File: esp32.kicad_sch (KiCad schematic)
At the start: 52 parts, among them J2 Conn_01x05, SW1 Reset, SW2 BOOT, U15 MPR121QR2, U8 ESP32-S3R8, U9 W25Q128JVSIQ, Y1 40MHz

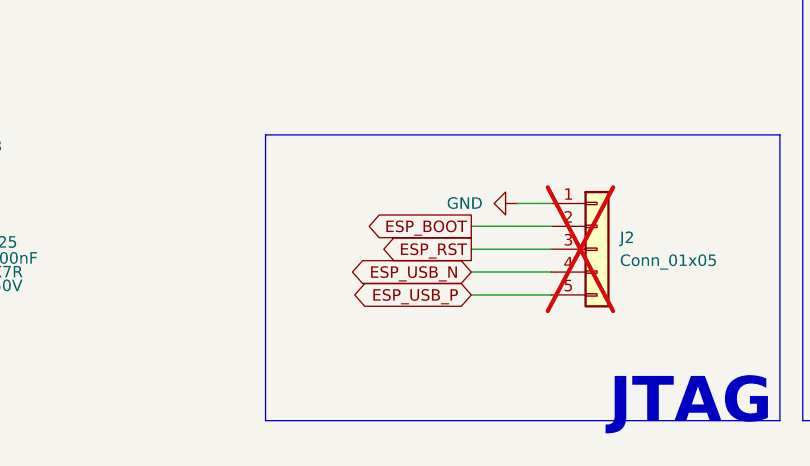
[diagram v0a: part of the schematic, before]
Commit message: WiP update
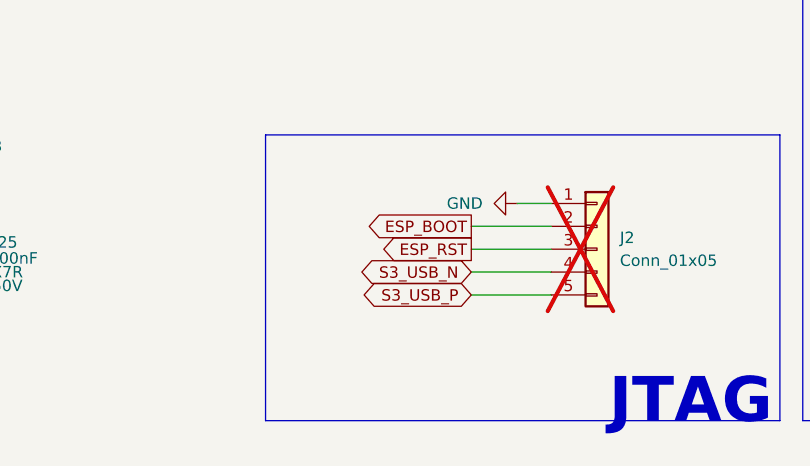
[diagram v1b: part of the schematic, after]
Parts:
- TP14, TP15, TP16: footprint TestPoint:TestPoint_Pad_2.5x2.5mm -> Onju:Touchpad
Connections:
- net ESP_USB_N is gone; now on net S3_USB_N: J2.4 (Pin_4)
- net ESP_USB_P is gone; now on net S3_USB_P: J2.5 (Pin_5)
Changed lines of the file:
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@@
 		)
 	)
-	(global_label "ESP_USB_N"
+	(global_label "S3_USB_N"
 		(shape bidirectional)
 		(at 106.68 264.16 180)
@@
 		)
 		(property "Intersheetrefs" "${INTERSHEET_REFS}"
-			(at 91.8793 264.16 0)
+			(at 93.0888 264.16 0)
 			(effects
 				(font
@@
 		)
 	)
-	(global_label "ESP_USB_P"
+	(global_label "S3_USB_P"
 		(shape bidirectional)
 		(at 106.68 266.7 180)
@@
 		)
 		(property "Intersheetrefs" "${INTERSHEET_REFS}"
-			(at 91.9398 266.7 0)
+			(at 93.1493 266.7 0)
 			(effects
 				(font
@@
 			)
 		)
-		(property "Footprint" "TestPoint:TestPoint_Pad_2.5x2.5mm"
+		(property "Footprint" "Onju:Touchpad"
 			(at 280.67 250.19 0)
 			(effects
@@
 			)
 		)
-		(property "Footprint" "TestPoint:TestPoint_Pad_2.5x2.5mm"
+		(property "Footprint" "Onju:Touchpad"
 			(at 280.67 247.65 0)
 			(effects
@@
 			)
 		)
-		(property "Footprint" "TestPoint:TestPoint_Pad_2.5x2.5mm"
+		(property "Footprint" "Onju:Touchpad"
 			(at 280.67 252.73 0)
 			(effects
